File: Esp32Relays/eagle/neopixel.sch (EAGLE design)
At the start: 20 parts, among them J1 Audio2, J3 AUDIO_JACK_3.5MM_PTH, J4 AUDIO_JACK_3.5MM_PTH, U1 CD4066BE

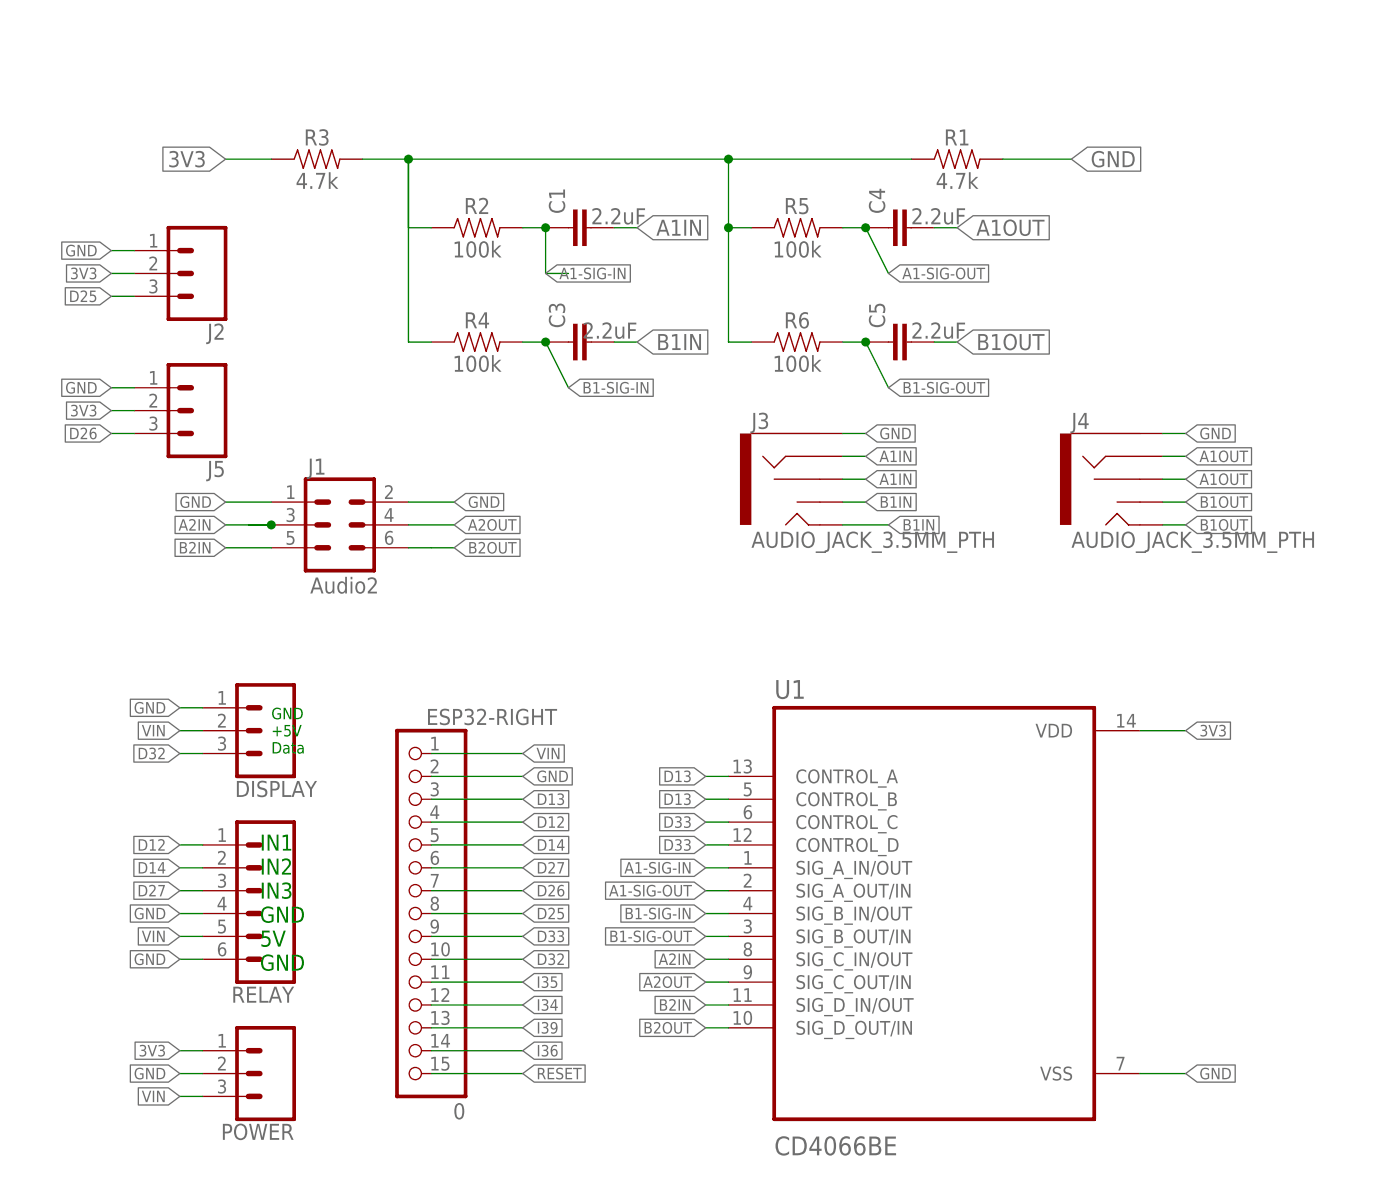
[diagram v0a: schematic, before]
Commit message: Schematic update
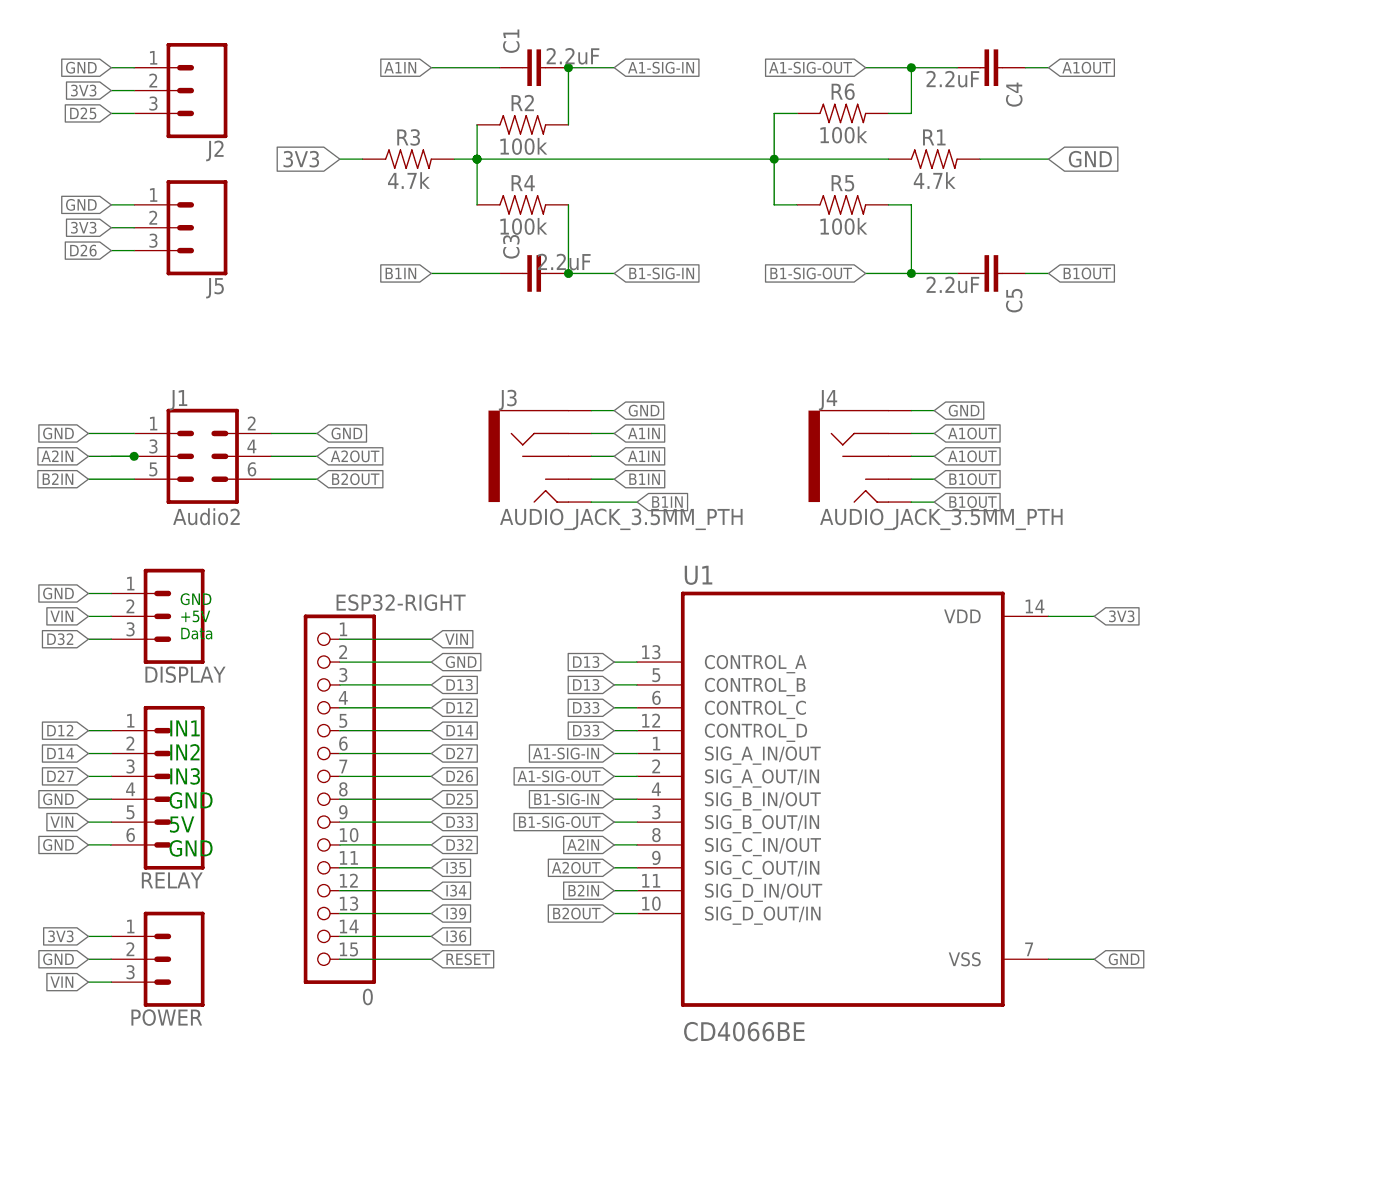
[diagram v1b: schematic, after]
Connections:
- net A1-SIG-IN: now also C1.2; no longer C1.1
- net A1-SIG-OUT: now also C4.2, R6.2; no longer C4.1, R5.2
- net A1IN: now also C1.1; no longer C1.2
- net A1OUT: now also C4.1; no longer C4.2
- net B1-SIG-IN: now also C3.2; no longer C3.1
- net B1-SIG-OUT: now also C5.2, R5.2; no longer C5.1, R6.2
- net B1IN: now also C3.1; no longer C3.2
- net B1OUT: now also C5.1; no longer C5.2
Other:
- moved on the sheet: C1, C3, C4, C5, DISPLAY, ESP32-RIGHT, J1, J2, J3, J4, J5, POWER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
